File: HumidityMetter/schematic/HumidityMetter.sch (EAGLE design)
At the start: 66 parts, among them IC1 LM317, IC2 LM317, IC3 STM32F103C8T6, IC4 AM2320, J1 0, J2 0, J3 0, J4 0, K1 POWER_ON, T1 BSS84, T2 BC847, X1 +9V, X2 GND, X3 ISP

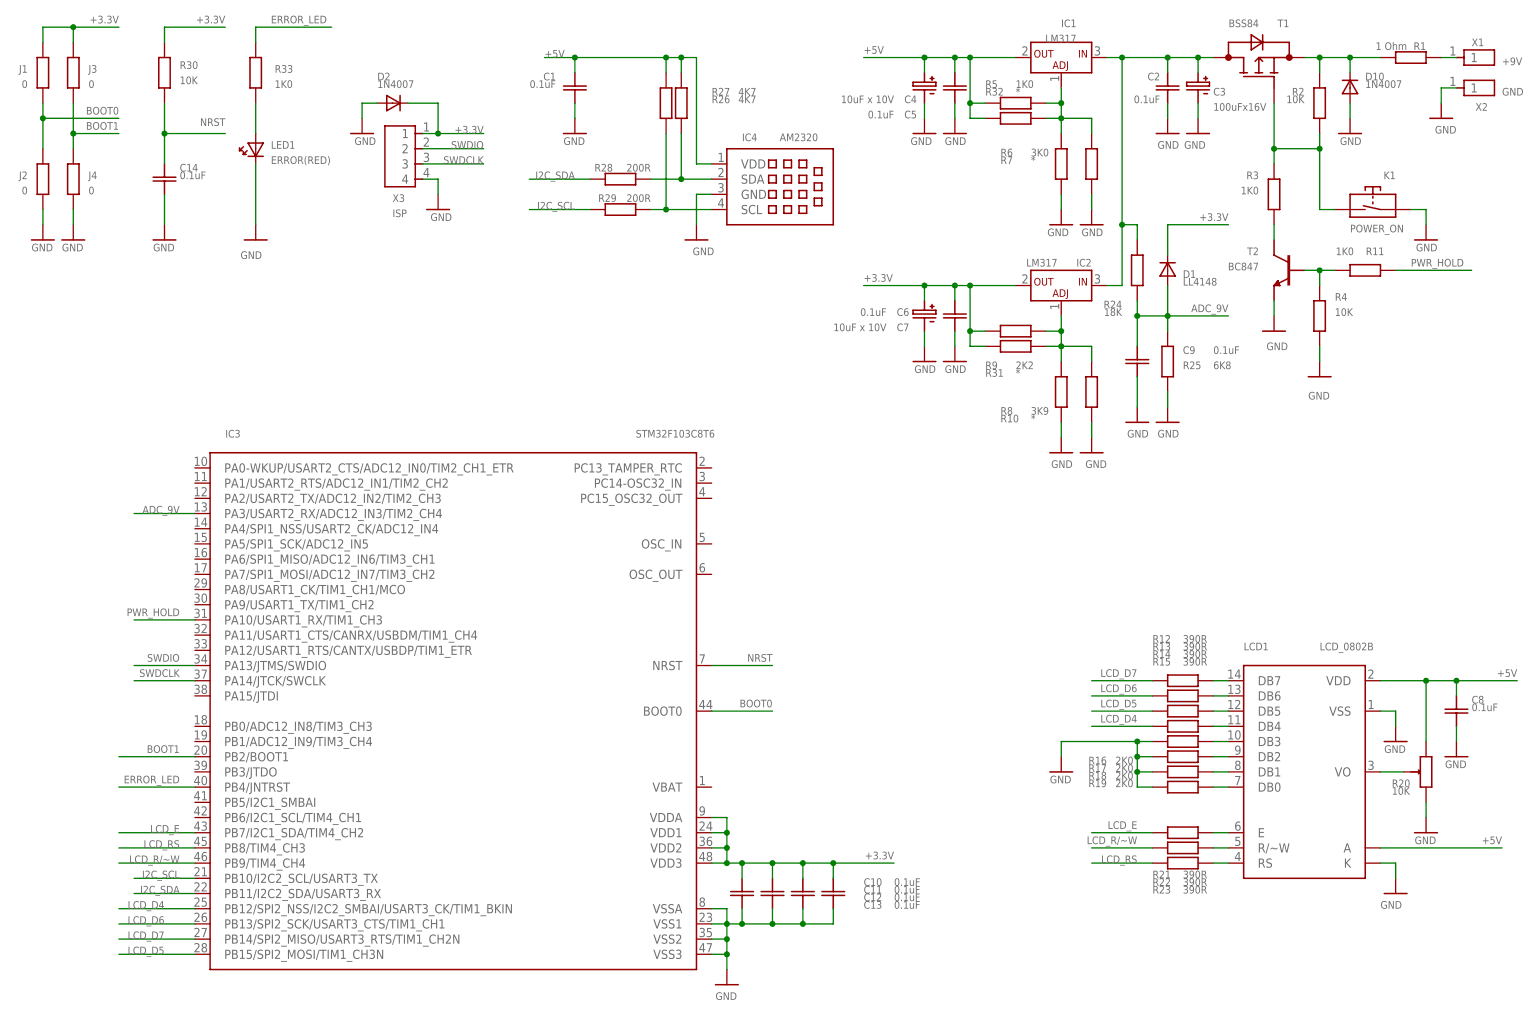
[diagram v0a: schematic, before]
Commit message: Humidity metter. Add key reading and switching between temp, humidity, preassure and battery voltage(dummy).
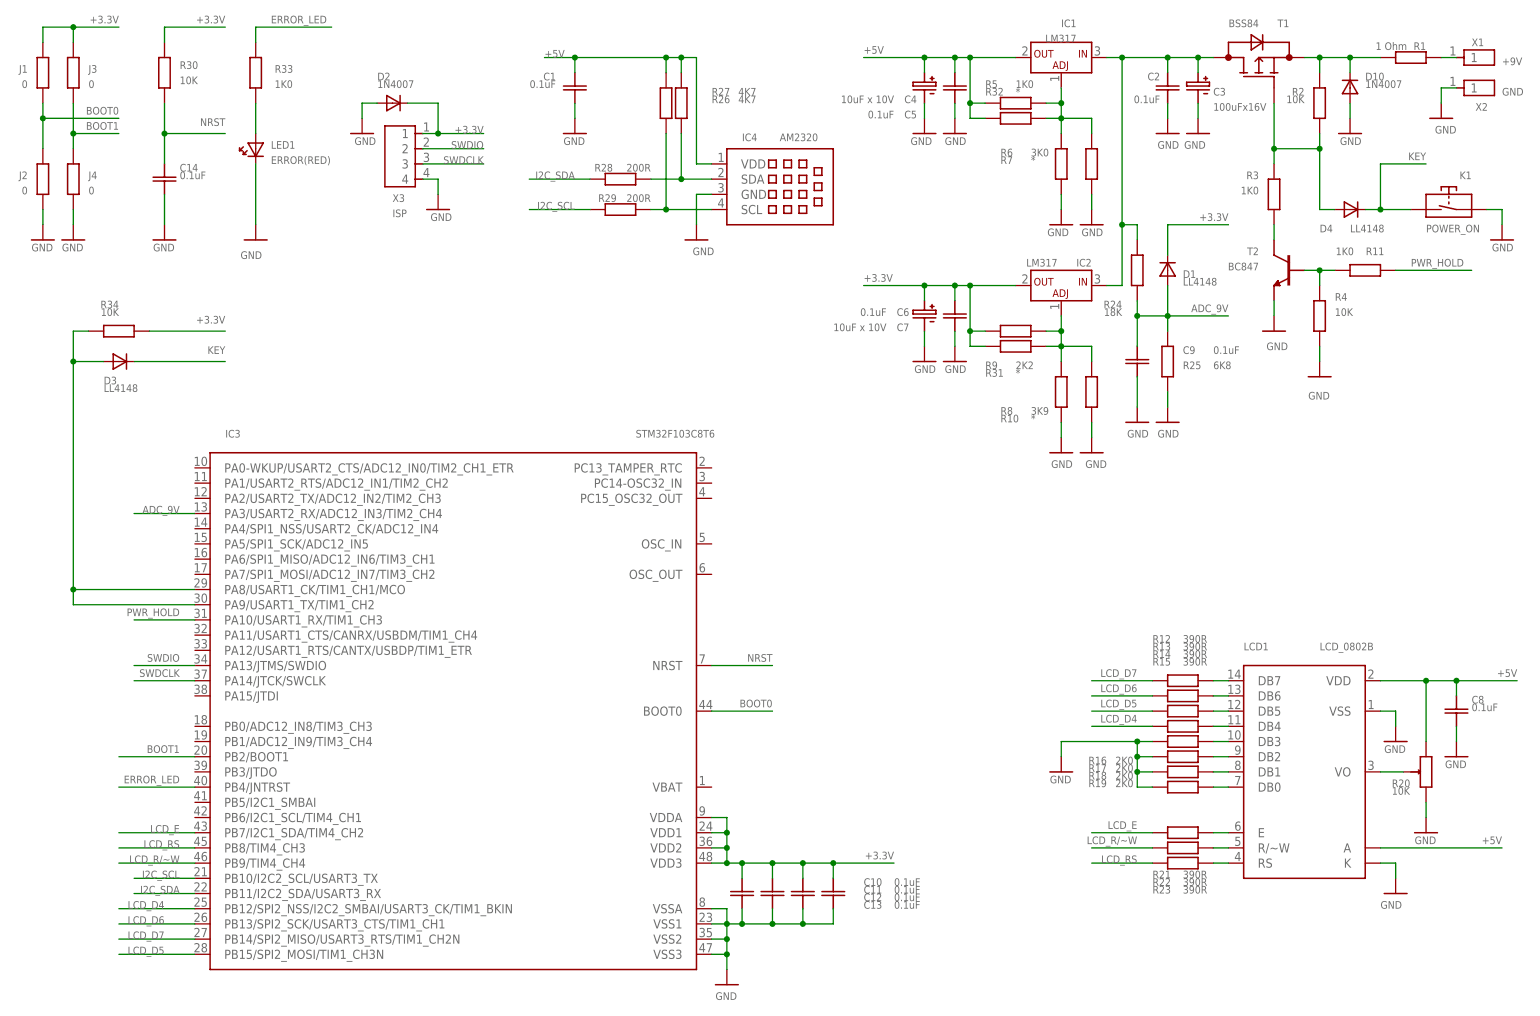
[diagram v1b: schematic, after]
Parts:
- added D3, D4: LL4148, __MyCommonLib1:LL4147SOD-80
- added R34: 10K, __MyCommonLib1:RSMD_0805
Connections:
- new net KEY: D3.CATHODE, D4.CATHODE, K1.2
- new net N$24: D3.ANODE, IC3.PA8/USART1_CK/TIM1_CH1/MCO, IC3.PA9/USART1_TX/TIM1_CH2, R34.PIN0
- net +3.3V: now also R34.PIN1
- net N$3: now also D4.ANODE; no longer K1.2
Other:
- moved on the sheet: K1
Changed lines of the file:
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@@
 <setting verticaltext="up"/>
 </settings>
-<grid distance="0.1" unitdist="inch" unit="inch" style="lines" multiple="1" display="no" altdistance="0.01" altunitdist="inch" altunit="inch"/>
+<grid distance="0.025" unitdist="inch" unit="inch" style="lines" multiple="4" display="yes" altdistance="0.01" altunitdist="inch" altunit="inch"/>
 <layers>
 <layer number="1" name="Top" color="4" fill="1" visible="no" active="no"/>
@@
 <part name="D2" library="__MyCommonLib1" deviceset="1N4001" device="DO-41_10MM" value="1N4007"/>
 <part name="GND31" library="supply1" deviceset="GND" device=""/>
+<part name="D3" library="__MyCommonLib1" deviceset="LL4147" device="SOD-80" value="LL4148"/>
+<part name="R34" library="__MyCommonLib1" deviceset="R" device="SMD_0805" value="10K"/>
+<part name="D4" library="__MyCommonLib1" deviceset="LL4147" device="SOD-80" value="LL4148"/>
 </parts>
 <sheets>
@@
 <attribute name="VALUE" x="210.82" y="144.78" size="1.27" layer="96" font="vector" ratio="20" rot="MR0"/>
 </instance>
-<instance part="GND2" gate="1" x="238.76" y="137.16" smashed="yes" rot="MR0">
-<attribute name="VALUE" x="240.665" y="135.255" size="1.27" layer="96" font="vector" ratio="20" rot="MR0"/>
-</instance>
-<instance part="K1" gate="G$1" x="229.87" y="142.24" smashed="yes" rot="MR0">
-<attribute name="NAME" x="233.68" y="147.32" size="1.27" layer="95" font="vector" ratio="20" rot="MR0"/>
-<attribute name="VALUE" x="226.06" y="139.7" size="1.27" layer="96" font="vector" ratio="20" rot="MR180"/>
+<instance part="GND2" gate="1" x="251.46" y="137.16" smashed="yes" rot="MR0">
+<attribute name="VALUE" x="253.365" y="135.255" size="1.27" layer="96" font="vector" ratio="20" rot="MR0"/>
+</instance>
+<instance part="K1" gate="G$1" x="242.57" y="142.24" smashed="yes" rot="MR0">
+<attribute name="NAME" x="246.38" y="147.32" size="1.27" layer="95" font="vector" ratio="20" rot="MR0"/>
+<attribute name="VALUE" x="238.76" y="139.7" size="1.27" layer="96" font="vector" ratio="20" rot="MR180"/>
 </instance>
 <instance part="T2" gate="T$1" x="215.9" y="132.08" smashed="yes" rot="MR0">
@@
 <instance part="GND31" gate="1" x="60.96" y="154.94" smashed="yes">
 <attribute name="VALUE" x="59.69" y="153.035" size="1.27" layer="96" font="vector" ratio="20"/>
+</instance>
+<instance part="D3" gate="D1" x="20.32" y="116.84" smashed="yes" rot="R270">
+<attribute name="NAME" x="17.78" y="113.03" size="1.27" layer="95" font="vector" ratio="20"/>
+<attribute name="VALUE" x="17.78" y="111.76" size="1.27" layer="96" font="vector" ratio="20"/>
+</instance>
+<instance part="R34" gate="R$1" x="20.32" y="121.92" smashed="yes" rot="R270">
+<attribute name="NAME" x="20.32" y="127" size="1.27" layer="95" font="vector" ratio="20" rot="R180"/>
+<attribute name="VALUE" x="20.32" y="125.73" size="1.27" layer="96" font="vector" ratio="20" rot="R180"/>
+</instance>
+<instance part="D4" gate="D1" x="226.06" y="142.24" smashed="yes" rot="R270">
+<attribute name="NAME" x="220.98" y="138.43" size="1.27" layer="95" font="vector" ratio="20"/>
+<attribute name="VALUE" x="226.06" y="138.43" size="1.27" layer="96" font="vector" ratio="20"/>
 </instance>
 </instances>
@@
 <pinref part="K1" gate="G$1" pin="1"/>
 <pinref part="GND2" gate="1" pin="GND"/>
-<wire x1="236.22" y1="142.24" x2="238.76" y2="142.24" width="0.1524" layer="91"/>
-<wire x1="238.76" y1="142.24" x2="238.76" y2="139.7" width="0.1524" layer="91"/>
+<wire x1="248.92" y1="142.24" x2="251.46" y2="142.24" width="0.1524" layer="91"/>
+<wire x1="251.46" y1="142.24" x2="251.46" y2="139.7" width="0.1524" layer="91"/>
 </segment>
 <segment>
@@
 <wire x1="213.36" y1="160.02" x2="213.36" y2="152.4" width="0.1524" layer="91"/>
 <junction x="213.36" y="152.4"/>
-<pinref part="K1" gate="G$1" pin="2"/>
-<wire x1="223.52" y1="142.24" x2="220.98" y2="142.24" width="0.1524" layer="91"/>
 <wire x1="220.98" y1="142.24" x2="220.98" y2="152.4" width="0.1524" layer="91"/>
 <junction x="220.98" y="152.4"/>
+<pinref part="D4" gate="D1" pin="ANODE"/>
+<wire x1="223.52" y1="142.24" x2="220.98" y2="142.24" width="0.1524" layer="91"/>
 </segment>
 </net>
@@
 <label x="149.86" y="34.925" size="1.27" layer="95" font="vector" ratio="20" rot="R180"/>
 </segment>
+<segment>
+<pinref part="R34" gate="R$1" pin="PIN1"/>
+<wire x1="25.4" y1="121.92" x2="38.1" y2="121.92" width="0.1524" layer="91"/>
+<label x="38.1" y="124.46" size="1.27" layer="95" font="vector" ratio="20" rot="R180"/>
+</segment>
 </net>
 <net name="PWR_HOLD" class="0">
@@
 </segment>
 </net>
+<net name="N$24" class="0">
+<segment>
+<pinref part="R34" gate="R$1" pin="PIN0"/>
+<wire x1="15.24" y1="121.92" x2="12.7" y2="121.92" width="0.1524" layer="91"/>
+<wire x1="12.7" y1="121.92" x2="12.7" y2="116.84" width="0.1524" layer="91"/>
+<pinref part="D3" gate="D1" pin="ANODE"/>
+<wire x1="12.7" y1="116.84" x2="17.78" y2="116.84" width="0.1524" layer="91"/>
+<pinref part="IC3" gate="G$1" pin="PA8/USART1_CK/TIM1_CH1/MCO"/>
+<wire x1="12.7" y1="116.84" x2="12.7" y2="78.74" width="0.1524" layer="91"/>
+<wire x1="12.7" y1="78.74" x2="33.02" y2="78.74" width="0.1524" layer="91"/>
+<pinref part="IC3" gate="G$1" pin="PA9/USART1_TX/TIM1_CH2"/>
+<wire x1="33.02" y1="76.2" x2="12.7" y2="76.2" width="0.1524" layer="91"/>
+<wire x1="12.7" y1="76.2" x2="12.7" y2="78.74" width="0.1524" layer="91"/>
+<junction x="12.7" y="78.74"/>
+<junction x="12.7" y="116.84"/>
+</segment>
+</net>
+<net name="KEY" class="0">
+<segment>
+<pinref part="D3" gate="D1" pin="CATHODE"/>
+<wire x1="22.86" y1="116.84" x2="38.1" y2="116.84" width="0.1524" layer="91"/>
+<label x="38.1" y="119.38" size="1.27" layer="95" font="vector" ratio="20" rot="R180"/>
+</segment>
+<segment>
+<pinref part="K1" gate="G$1" pin="2"/>
+<pinref part="D4" gate="D1" pin="CATHODE"/>
+<wire x1="236.22" y1="142.24" x2="231.14" y2="142.24" width="0.1524" layer="91"/>
+<wire x1="231.14" y1="142.24" x2="228.6" y2="142.24" width="0.1524" layer="91"/>
+<wire x1="231.14" y1="142.24" x2="231.14" y2="149.86" width="0.1524" layer="91"/>
+<wire x1="231.14" y1="149.86" x2="238.76" y2="149.86" width="0.1524" layer="91"/>
+<junction x="231.14" y="142.24"/>
+<label x="238.76" y="151.765" size="1.27" layer="95" font="vector" ratio="20" rot="R180"/>
+</segment>
+</net>
